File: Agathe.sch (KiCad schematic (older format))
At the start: 153 parts, among them SW1 SW_Push, U1 ATmega32U4-AU, U2 PRTR5V0U2X, Y1 Crystal_GND24_Small

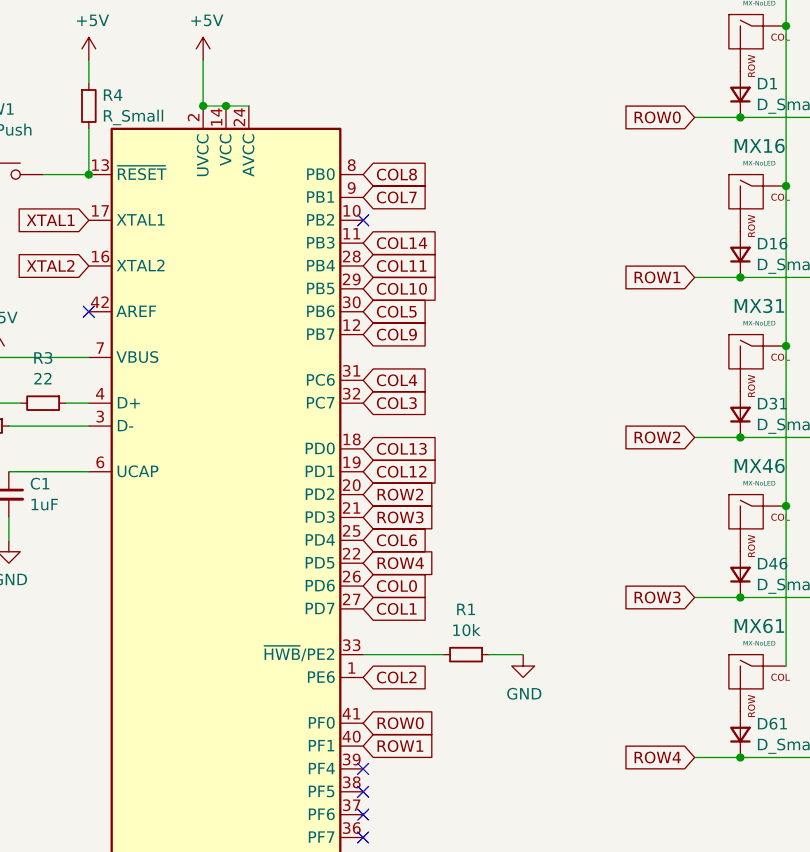
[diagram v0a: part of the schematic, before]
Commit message: Route everything
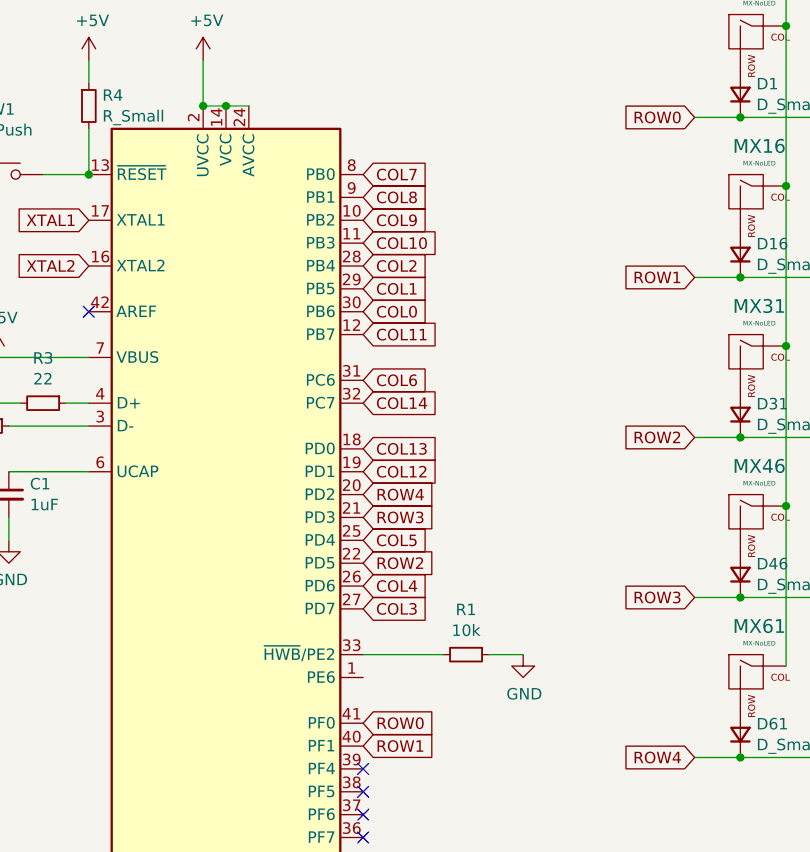
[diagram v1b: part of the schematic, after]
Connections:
- net COL0: now also U1.30 (PB6); no longer U1.26 (PD6)
- net COL1: now also U1.29 (PB5); no longer U1.27 (PD7)
- net COL10: now also U1.11 (PB3); no longer U1.29 (PB5)
- net COL11: now also U1.12 (PB7); no longer U1.28 (PB4)
- net COL14: now also U1.32 (PC7); no longer U1.11 (PB3)
- net COL2: now also U1.28 (PB4); no longer U1.1 (PE6)
- net COL3: now also U1.27 (PD7); no longer U1.32 (PC7)
- net COL4: now also U1.26 (PD6); no longer U1.31 (PC6)
- net COL5: now also U1.25 (PD4); no longer U1.30 (PB6)
- net COL6: now also U1.31 (PC6); no longer U1.25 (PD4)
- net COL7: now also U1.8 (PB0); no longer U1.9 (PB1)
- net COL8: now also U1.9 (PB1); no longer U1.8 (PB0)
- net COL9: now also U1.10 (PB2); no longer U1.12 (PB7)
- net ROW2: now also U1.22 (PD5); no longer U1.20 (PD2)
- net ROW4: now also U1.20 (PD2); no longer U1.22 (PD5)
- no-connect marks 8 -> 7
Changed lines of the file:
@@
 $EndComp
 NoConn ~ 5600 6300
+Text GLabel 2850 1850 2    50   Input ~ 0
+COL8
 Text GLabel 2850 1750 2    50   Input ~ 0
-COL8
-Text GLabel 2850 1850 2    50   Input ~ 0
 COL7
-Text GLabel 2850 2050 2    50   Input ~ 0
+Text GLabel 2850 2750 2    50   Input ~ 0
 COL14
-Text GLabel 2850 2150 2    50   Input ~ 0
-COL11
-Text GLabel 2850 2250 2    50   Input ~ 0
-COL10
-Text GLabel 2850 2350 2    50   Input ~ 0
+Text GLabel 2850 3350 2    50   Input ~ 0
 COL5
-Text GLabel 2850 2450 2    50   Input ~ 0
+Text GLabel 2850 1950 2    50   Input ~ 0
 COL9
-Text GLabel 2850 2650 2    50   Input ~ 0
+Text GLabel 2850 3550 2    50   Input ~ 0
 COL4
-Text GLabel 2850 2750 2    50   Input ~ 0
+Text GLabel 2850 3650 2    50   Input ~ 0
 COL3
 Text GLabel 2850 4150 2    50   Input ~ 0
@@
 Text GLabel 2850 4250 2    50   Input ~ 0
 ROW1
-Text GLabel 2850 3150 2    50   Input ~ 0
+Text GLabel 2850 3450 2    50   Input ~ 0
 ROW2
-Text GLabel 2850 3250 2    50   Input ~ 0
-ROW3
-Text GLabel 2850 3350 2    50   Input ~ 0
-COL6
-Text GLabel 2850 3450 2    50   Input ~ 0
-ROW4
 Text GLabel 2850 2950 2    50   Input ~ 0
 COL13
@@
 Text GLabel 2850 3050 2    50   Input ~ 0
 COL12
-Text GLabel 2850 3950 2    50   Input ~ 0
-COL2
-Text GLabel 2850 3550 2    50   Input ~ 0
+Text GLabel 2850 2350 2    50   Input ~ 0
 COL0
-Text GLabel 2850 3650 2    50   Input ~ 0
-COL1
 NoConn ~ 2850 4350
 NoConn ~ 2850 4450
@@
 NoConn ~ 2850 4650
 NoConn ~ 1650 2350
-NoConn ~ 2850 1950
 Wire Wire Line
 	10550 1800 10550 3200
@@
 	11000 3900 11000 2500
 Connection ~ 11000 2500
+Text GLabel 2850 3150 2    50   Input ~ 0
+ROW4
+Text GLabel 2850 3250 2    50   Input ~ 0
+ROW3
+Text GLabel 2850 2050 2    50   Input ~ 0
+COL10
+Text GLabel 2850 2450 2    50   Input ~ 0
+COL11
+Text GLabel 2850 2250 2    50   Input ~ 0
+COL1
+Text GLabel 2850 2150 2    50   Input ~ 0
+COL2
+Text GLabel 2850 2650 2    50   Input ~ 0
+COL6
 $EndSCHEMATC
